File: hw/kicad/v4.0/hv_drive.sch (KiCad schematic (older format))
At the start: 21 parts, among them P6 CONN_01X02, P8 CONN_01X03, U12 IRAM256a

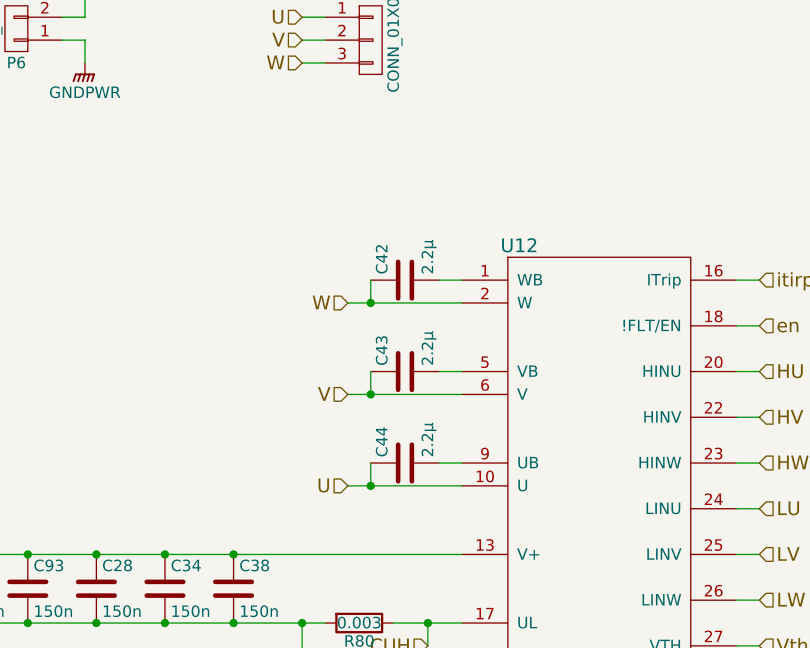
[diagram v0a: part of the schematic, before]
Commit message: added HW files
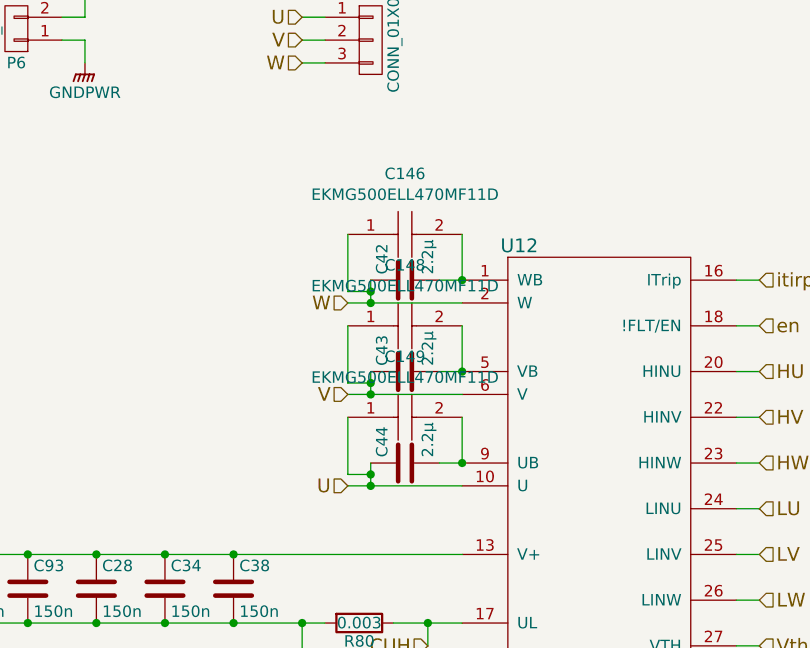
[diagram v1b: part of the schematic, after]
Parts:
- added C146, C148, C149: EKMG500ELL470MF11D, SamacSys_Parts:CAPPRD250W60D680H1250, symbol SamacSys_Parts:EKMG500ELL470MF11D
- C42, C43, C44: footprint stmbl:C_0603 -> stmbl:C_1206
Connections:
- net U: now also C149.1
- net V: now also C148.1
- net W: now also C146.1
- net at C42.2, U12.1 (WB): now also C146.2
- net at C43.2, U12.5 (VB): now also C148.2
- net at C44.2, U12.9 (UB): now also C149.2
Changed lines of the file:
@@
 EESchema Schematic File Version 4
-LIBS:stmbl_4.0-cache
-EELAYER 26 0
+EELAYER 30 0
 EELAYER END
 $Descr A4 11693 8268
@@
 F 0 "C42" H 5625 3150 50  0000 L CNN
 F 1 "2.2µ" H 5625 2950 50  0000 L CNN
-F 2 "stmbl:C_0603" H 5638 2900 30  0001 C CNN
+F 2 "stmbl:C_1206" H 5638 2900 30  0001 C CNN
 F 3 "" H 5600 3050 60  0000 C CNN
 F 4 "" H 5600 3050 60  0001 C CNN "InternalName"
@@
 F 0 "C43" H 5625 3550 50  0000 L CNN
 F 1 "2.2µ" H 5625 3350 50  0000 L CNN
-F 2 "stmbl:C_0603" H 5638 3300 30  0001 C CNN
+F 2 "stmbl:C_1206" H 5638 3300 30  0001 C CNN
 F 3 "" H 5600 3450 60  0000 C CNN
 F 4 "" H 5600 3450 60  0001 C CNN "InternalName"
@@
 	5350 3550 5450 3550
 Wire Wire Line
-	5450 3450 5450 3550
+	5450 3450 5450 3500
 Connection ~ 5450 3550
 $Comp
@@
 F 0 "C44" H 5625 3950 50  0000 L CNN
 F 1 "2.2µ" H 5625 3750 50  0000 L CNN
-F 2 "stmbl:C_0603" H 5638 3700 30  0001 C CNN
+F 2 "stmbl:C_1206" H 5638 3700 30  0001 C CNN
 F 3 "" H 5600 3850 60  0000 C CNN
 F 4 "" H 5600 3850 60  0001 C CNN "InternalName"
@@
 $EndComp
 Wire Wire Line
-	5850 3850 5750 3850
-Wire Wire Line
 	5350 3950 5450 3950
 Wire Wire Line
-	5450 3850 5450 3950
+	5450 3850 5450 3900
 Connection ~ 5450 3950
 $Comp
@@
 	7800 4550 7900 4550
 Wire Wire Line
-	5450 3050 5450 3150
+	5450 3050 5450 3100
 Wire Wire Line
 	5150 4550 5150 4750
@@
 Wire Wire Line
 	8100 4750 8400 4750
+$Comp
+L SamacSys_Parts:EKMG500ELL470MF11D C146
+U 1 1 5DF898C9
+P 5350 2850
+F 0 "C146" H 5600 3115 50  0000 C CNN
+F 1 "EKMG500ELL470MF11D" H 5600 3024 50  0000 C CNN
+F 2 "SamacSys_Parts:CAPPRD250W60D680H1250" H 5700 2900 50  0001 L CNN
+F 3 "https://componentsearchengine.com/Datasheets/1/EKMG500ELL470MF11D.pdf" H 5700 2800 50  0001 L CNN
+F 4 "UNITED CHEMI-CON - EKMG500ELL470MF11D - ALUMINUM ELECTROLYTIC CAPACITOR 47UF, 50V, 20%, RADIAL" H 5700 2700 50  0001 L CNN "Description"
+F 5 "12.5" H 5700 2600 50  0001 L CNN "Height"
+F 6 "661-EKMGG500ELL470MF" H 5700 2500 50  0001 L CNN "Mouser Part Number"
+F 7 "https://www.mouser.com/Search/Refine.aspx?Keyword=661-EKMGG500ELL470MF" H 5700 2400 50  0001 L CNN "Mouser Price/Stock"
+F 8 "United Chemi-Con" H 5700 2300 50  0001 L CNN "Manufacturer_Name"
+F 9 "EKMG500ELL470MF11D" H 5700 2200 50  0001 L CNN "Manufacturer_Part_Number"
+	1    5350 2850
+	1    0    0    -1
+$EndComp
+$Comp
+L SamacSys_Parts:EKMG500ELL470MF11D C148
+U 1 1 5DF8F912
+P 5350 3250
+F 0 "C148" H 5600 3515 50  0000 C CNN
+F 1 "EKMG500ELL470MF11D" H 5600 3424 50  0000 C CNN
+F 2 "SamacSys_Parts:CAPPRD250W60D680H1250" H 5700 3300 50  0001 L CNN
+F 3 "https://componentsearchengine.com/Datasheets/1/EKMG500ELL470MF11D.pdf" H 5700 3200 50  0001 L CNN
+F 4 "UNITED CHEMI-CON - EKMG500ELL470MF11D - ALUMINUM ELECTROLYTIC CAPACITOR 47UF, 50V, 20%, RADIAL" H 5700 3100 50  0001 L CNN "Description"
+F 5 "12.5" H 5700 3000 50  0001 L CNN "Height"
+F 6 "661-EKMGG500ELL470MF" H 5700 2900 50  0001 L CNN "Mouser Part Number"
+F 7 "https://www.mouser.com/Search/Refine.aspx?Keyword=661-EKMGG500ELL470MF" H 5700 2800 50  0001 L CNN "Mouser Price/Stock"
+F 8 "United Chemi-Con" H 5700 2700 50  0001 L CNN "Manufacturer_Name"
+F 9 "EKMG500ELL470MF11D" H 5700 2600 50  0001 L CNN "Manufacturer_Part_Number"
+	1    5350 3250
+	1    0    0    -1
+$EndComp
+$Comp
+L SamacSys_Parts:EKMG500ELL470MF11D C149
+U 1 1 5DF91ED9
+P 5350 3650
+F 0 "C149" H 5600 3915 50  0000 C CNN
+F 1 "EKMG500ELL470MF11D" H 5600 3824 50  0000 C CNN
+F 2 "SamacSys_Parts:CAPPRD250W60D680H1250" H 5700 3700 50  0001 L CNN
+F 3 "https://componentsearchengine.com/Datasheets/1/EKMG500ELL470MF11D.pdf" H 5700 3600 50  0001 L CNN
+F 4 "UNITED CHEMI-CON - EKMG500ELL470MF11D - ALUMINUM ELECTROLYTIC CAPACITOR 47UF, 50V, 20%, RADIAL" H 5700 3500 50  0001 L CNN "Description"
+F 5 "12.5" H 5700 3400 50  0001 L CNN "Height"
+F 6 "661-EKMGG500ELL470MF" H 5700 3300 50  0001 L CNN "Mouser Part Number"
+F 7 "https://www.mouser.com/Search/Refine.aspx?Keyword=661-EKMGG500ELL470MF" H 5700 3200 50  0001 L CNN "Mouser Price/Stock"
+F 8 "United Chemi-Con" H 5700 3100 50  0001 L CNN "Manufacturer_Name"
+F 9 "EKMG500ELL470MF11D" H 5700 3000 50  0001 L CNN "Manufacturer_Part_Number"
+	1    5350 3650
+	1    0    0    -1
+$EndComp
+Wire Wire Line
+	5850 3650 5850 3850
+Connection ~ 5850 3850
+Wire Wire Line
+	5850 3250 5850 3450
+Wire Wire Line
+	5750 3850 5850 3850
+Connection ~ 5850 3450
+Wire Wire Line
+	5850 2850 5850 3050
+Connection ~ 5850 3050
+Wire Wire Line
+	5350 2850 5350 3100
+Wire Wire Line
+	5350 3100 5450 3100
+Connection ~ 5450 3100
+Wire Wire Line
+	5450 3100 5450 3150
+Wire Wire Line
+	5350 3250 5350 3500
+Wire Wire Line
+	5350 3500 5450 3500
+Connection ~ 5450 3500
+Wire Wire Line
+	5450 3500 5450 3550
+Wire Wire Line
+	5350 3650 5350 3900
+Wire Wire Line
+	5350 3900 5450 3900
+Connection ~ 5450 3900
+Wire Wire Line
+	5450 3900 5450 3950
 $EndSCHEMATC
